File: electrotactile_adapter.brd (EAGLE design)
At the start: 29.6 x 16.7 mm, 16 parts, among them J3 PAD_SMD_L0.5_W1, J4 PAD_SMD_L0.5_W1, J5 PAD_SMD_L0.5_W1, J6 PAD_SMD_L0.5_W1, J7 1x33 Molex Connector, J8 1x33 Molex Connector

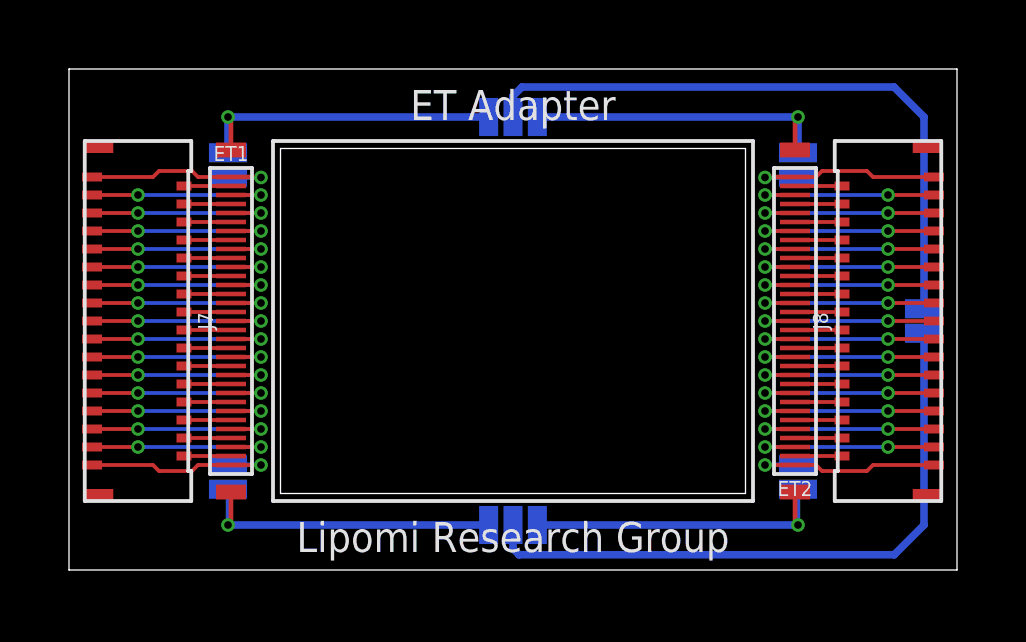
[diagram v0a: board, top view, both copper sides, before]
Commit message: update for Mickey.
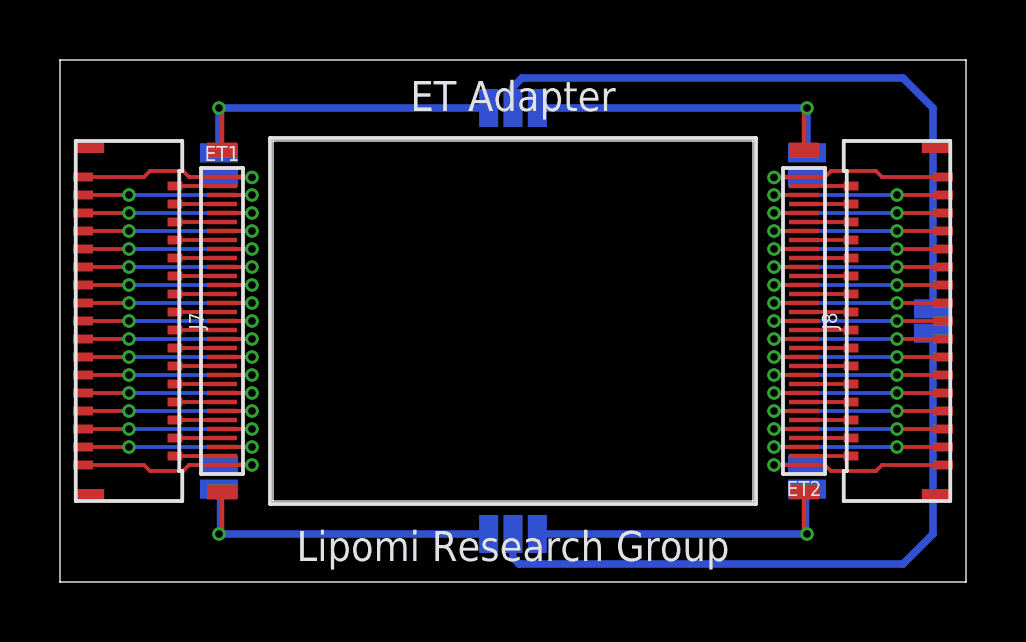
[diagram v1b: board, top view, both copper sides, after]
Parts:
- moved J7 0.30 mm to (-12.8, 0.00)
- moved J8 0.30 mm to (12.8, 0.00)
- moved JP2 0.30 mm to (-9.80, -5.20)
- moved JP3 0.30 mm to (-9.80, 5.20)
- moved JP4 0.30 mm to (9.80, 5.20)
- moved JP5 0.30 mm to (9.80, -5.20)
- moved JP7 0.30 mm to (14.0, 0.00)
- moved JP1 0.30 mm to (0.00, 7.10)
- moved JP6 0.30 mm to (0.00, -7.10)
- moved ET1 0.30 mm to (-9.70, 0.00)
- moved ET2 0.30 mm to (9.70, 0.00)
- moved J3 0.30 mm to (-9.70, 5.70)
- moved J4 0.30 mm to (-9.70, -5.70)
- moved J5 0.30 mm to (9.70, 5.70)
- moved J6 0.30 mm to (9.70, -5.70)
- renumbered U$2 to U$1
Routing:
- net N$70: track 11.0 -> 11.9 mm
- net N$69: track 11.0 -> 11.9 mm
- net N$68: track 11.0 -> 11.9 mm
- net N$34: track 11.0 -> 11.9 mm
- net N$71: track 21.4 -> 22.0 mm
- net N$72: track 21.3 -> 21.9 mm
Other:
- board size 29.6 x 16.7 mm -> 30.2 x 17.4 mm
